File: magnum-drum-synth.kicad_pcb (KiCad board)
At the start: 2 copper layers, 143.8 x 103.8 mm, 148 parts, among them J1 Input1, J2 Input1, J3 Trig_In, J4 Freq_CV, J5 Decay_CV, J6 Audio_Out, J7 Euro_Power, Q1 2N3904, Q2 2N3904, Q3 2N3904, Q4 2N3906, Q5 2N3906, Q6 2N3906, SW1 SW_SPDT, U1 HEF4093B, U2 TL072, U3 TL074, U4 LM13700, U5 LM13700, U6 LM13700

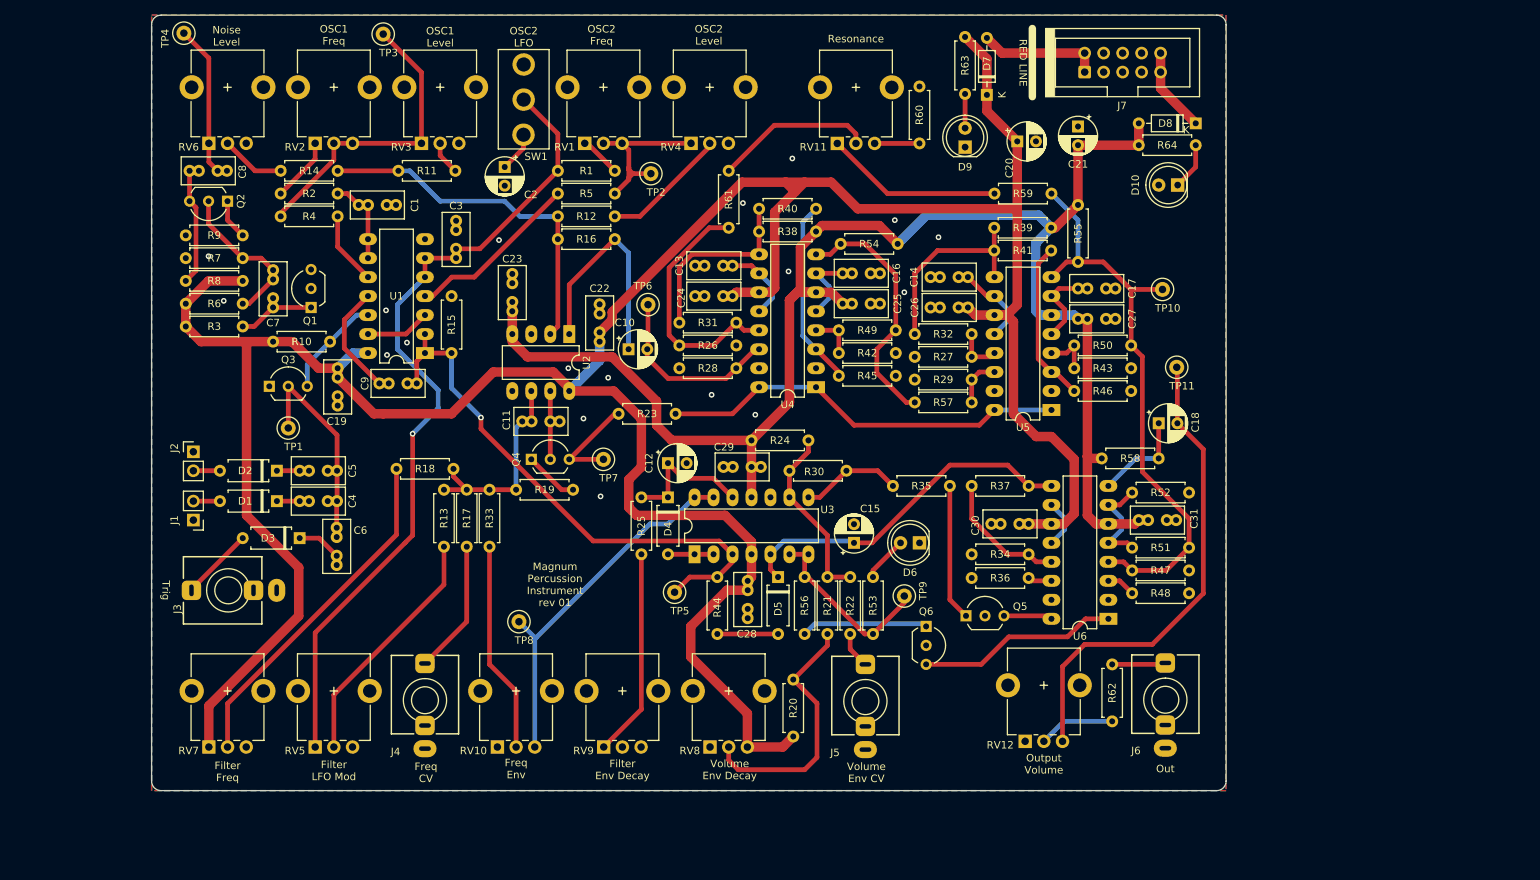
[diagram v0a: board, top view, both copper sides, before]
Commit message: Creating rev02
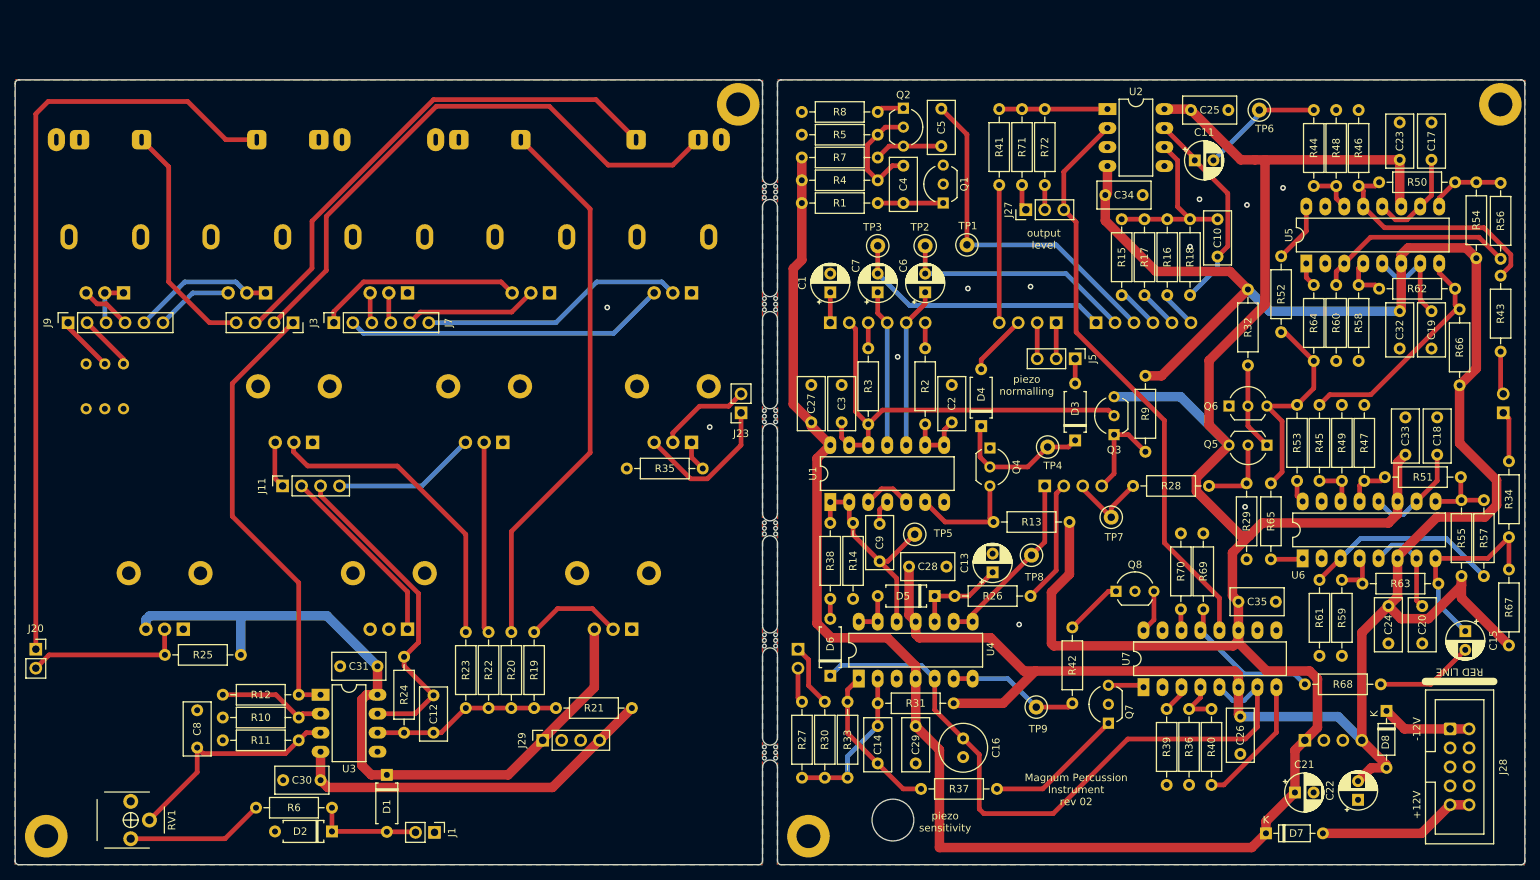
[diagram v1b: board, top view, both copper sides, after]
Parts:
- removed D10, D9: LED, LED_THT:LED_D5.0mm
- removed TP10, TP11: TestPoint, TestPoint:TestPoint_Loop_D2.50mm_Drill1.0mm_LowProfile
- added C32: 100nF (X7R), Rumblesan_Footprints:C_Rect_L7.0mm_W3.5mm_P5.00mm, F.Cu at (215.3, 65.9)
- added C33: 100nF (X7R), Rumblesan_Footprints:C_Rect_L7.0mm_W3.5mm_P5.00mm, F.Cu at (216.0, 80.2)
- added C34: 100nF (X7R), Rumblesan_Footprints:C_Rect_L7.0mm_W3.5mm_P5.00mm, F.Cu at (180.9, 45.4)
- added C35: 100nF (X7R), Rumblesan_Footprints:C_Rect_L7.0mm_W3.5mm_P5.00mm, F.Cu at (193.7, 99.8)
- added H1: MouseBite, Panelization:mouse-bite-2mm-slot, F.Cu at (131.0, 105.0)
- added H10: MountingHole_Pad, MountingHole:MountingHole_3.2mm_M3_ISO7380_Pad, F.Cu at (126.7, 33.3)
- added H2: MouseBite, Panelization:mouse-bite-2mm-slot, F.Cu at (131.0, 45.0)
- added H3: MouseBite, Panelization:mouse-bite-2mm-slot, F.Cu at (131.0, 75.0)
- added H4: MouseBite, Panelization:mouse-bite-2mm-slot, F.Cu at (131.0, 60.0)
- added H5: MouseBite, Panelization:mouse-bite-2mm-slot, F.Cu at (131.0, 120.0)
- added H6: MouseBite, Panelization:mouse-bite-2mm-slot, F.Cu at (131.0, 90.0)
- added H7: MountingHole_Pad, MountingHole:MountingHole_3.2mm_M3_ISO7380_Pad, F.Cu at (228.7, 33.3)
- added H8: MountingHole_Pad, MountingHole:MountingHole_3.2mm_M3_ISO7380_Pad, F.Cu at (136.1, 131.2)
- added H9: MountingHole_Pad, MountingHole:MountingHole_3.2mm_M3_ISO7380_Pad, F.Cu at (34.2, 131.2)
- added J10: Filter_Mod_Main, Connector_PinSocket_2.54mm:PinSocket_1x04_P2.54mm_Vertical, B.Cu at (167.8, 84.3)
- added J11: Filter_Mod_Ctrl, Connector_PinSocket_2.54mm:PinSocket_1x04_P2.54mm_Vertical, F.Cu at (65.8, 84.3)
- added J12: Freq_CV, EurorackBasics:Jack_3.5mm_QingPu_WQP-PJ398SM_Vertical, B.Cu at (92.8, 38.0)
- added J18: Decay_CV, EurorackBasics:Jack_3.5mm_QingPu_WQP-PJ398SM_Vertical, B.Cu at (67.2, 38.0)
- added J20: Amp_Decay_Ctrl, Connector_PinSocket_2.54mm:PinSocket_1x02_P2.54mm_Vertical, F.Cu at (32.8, 106.2)
- added J21: Amp_Decay_Main, Connector_PinHeader_2.54mm:PinHeader_1x02_P2.54mm_Vertical, B.Cu at (134.7, 106.2)
- added J22: Res_Main, Connector_PinHeader_2.54mm:PinHeader_1x02_P2.54mm_Vertical, B.Cu at (229.1, 74.5)
- added J23: Res_Ctrl, Connector_PinSocket_2.54mm:PinSocket_1x02_P2.54mm_Vertical, F.Cu at (127.1, 74.5)
- added J26: Audio_Out, EurorackBasics:Jack_3.5mm_QingPu_WQP-PJ398SM_Vertical, B.Cu at (42.0, 38.0)
- added J27: LevelSelect, Connector_PinHeader_2.54mm:PinHeader_1x03_P2.54mm_Vertical, F.Cu at (165.2, 47.4)
- added J28: Eurorack_Power_Small, EurorackBasics:Eurorack_PowerHeader_2x05_P2.54mm_Shrouded, F.Cu at (222.0, 116.8)
- added J29: POWER_CTRL, Connector_PinSocket_2.54mm:PinSocket_1x04_P2.54mm_Vertical, F.Cu at (100.6, 118.4)
- added J30: POWER_MAIN, Connector_PinHeader_2.54mm:PinHeader_1x04_P2.54mm_Vertical, B.Cu at (202.6, 118.4)
- added J8: Osc_Freq_Main, Connector_PinHeader_2.54mm:PinHeader_1x06_P2.54mm_Vertical, B.Cu at (139.1, 62.5)
- added J9: Osc_Freq_Ctrl, Connector_PinSocket_2.54mm:PinSocket_1x06_P2.54mm_Vertical, F.Cu at (37.1, 62.5)
- added Q7: 2N3906, Package_TO_SOT_THT:TO-92_Inline_Wide, F.Cu at (176.3, 116.1)
- added Q8: 2N3906, Package_TO_SOT_THT:TO-92_Inline_Wide, F.Cu at (177.3, 98.4)
- added R65: 21k, Rumblesan_Footprints:Resistor_THT_L6.3mm_D2.5mm_P10.16mm_Horizontal, F.Cu at (198.0, 94.1)
- added R66: 10k, Rumblesan_Footprints:Resistor_THT_L6.3mm_D2.5mm_P10.16mm_Horizontal, F.Cu at (223.3, 60.7)
- added R67: 10k, Rumblesan_Footprints:Resistor_THT_L6.3mm_D2.5mm_P10.16mm_Horizontal, F.Cu at (229.9, 95.5)
- added R68: 100k, Rumblesan_Footprints:Resistor_THT_L6.3mm_D2.5mm_P10.16mm_Horizontal, F.Cu at (212.7, 110.9)
- added R69: 220r, Rumblesan_Footprints:Resistor_THT_L6.3mm_D2.5mm_P10.16mm_Horizontal, F.Cu at (189.0, 100.8)
- added R70: 220r, Rumblesan_Footprints:Resistor_THT_L6.3mm_D2.5mm_P10.16mm_Horizontal, F.Cu at (186.0, 100.8)
- added R71: 18k, Rumblesan_Footprints:Resistor_THT_L6.3mm_D2.5mm_P10.16mm_Horizontal, F.Cu at (164.7, 44.1)
- added R72: 4k7, Rumblesan_Footprints:Resistor_THT_L6.3mm_D2.5mm_P10.16mm_Horizontal, F.Cu at (167.8, 44.1)
- added U7: LM13700, Package_DIP:DIP-16_W7.62mm_LongPads, F.Cu at (181.0, 111.3)
- C1, C7: value 47nF -> 1uF; footprint Rumblesan_Footprints:C_Rect_L7.0mm_W3.5mm_P2.50mm_P5.00mm -> Capacitor_THT:CP_Radial_D5.0mm_P2.50mm
- C10: value 10uF -> 22pF; footprint Capacitor_THT:CP_Radial_D5.0mm_P2.50mm -> Rumblesan_Footprints:C_Rect_L7.0mm_W3.5mm_P5.00mm
- C11: value 47pF -> 10uF; footprint Rumblesan_Footprints:C_Rect_L7.0mm_W3.5mm_P2.50mm_P5.00mm -> Capacitor_THT:CP_Radial_D5.0mm_P2.50mm
- C12: value 10uF -> 10nF; footprint Capacitor_THT:CP_Radial_D5.0mm_P2.50mm -> Rumblesan_Footprints:C_Rect_L7.0mm_W3.5mm_P5.00mm
- C13: value 1nF -> 10uF; footprint Rumblesan_Footprints:C_Rect_L7.0mm_W3.5mm_P2.50mm_P5.00mm -> Capacitor_THT:CP_Radial_D5.0mm_P2.50mm
- C14: value 1nF -> 22pF; footprint Rumblesan_Footprints:C_Rect_L7.0mm_W3.5mm_P2.50mm_P5.00mm -> Rumblesan_Footprints:C_Rect_L7.0mm_W3.5mm_P5.00mm
- C15: value 1uF -> 10uF
- C16: value 1nF -> 1uF; footprint Rumblesan_Footprints:C_Rect_L7.0mm_W3.5mm_P2.50mm_P5.00mm -> Capacitor_THT:C_Radial_D6.3mm_H7.0mm_P2.50mm
- C17: value 1nF -> 150pF (poly); footprint Rumblesan_Footprints:C_Rect_L7.0mm_W3.5mm_P2.50mm_P5.00mm -> Rumblesan_Footprints:C_Rect_L7.0mm_W3.5mm_P5.00mm
- C18: value 10uF -> 150pF (poly); footprint Capacitor_THT:CP_Radial_D5.0mm_P2.50mm -> Rumblesan_Footprints:C_Rect_L7.0mm_W3.5mm_P5.00mm
- C19: value 100nF (X7R) -> 150pF (poly); footprint Rumblesan_Footprints:C_Rect_L7.0mm_W3.5mm_P2.50mm_P5.00mm -> Rumblesan_Footprints:C_Rect_L7.0mm_W3.5mm_P5.00mm
- C2: value 1uF -> 47nF; footprint Capacitor_THT:CP_Radial_D5.0mm_P2.50mm -> Rumblesan_Footprints:C_Rect_L7.0mm_W3.5mm_P5.00mm
- C20: value 1uF -> 150pF (poly); footprint Capacitor_THT:CP_Radial_D5.0mm_P2.50mm -> Rumblesan_Footprints:C_Rect_L7.0mm_W3.5mm_P5.00mm
- C22: value 100nF (X7R) -> 1uF; footprint Rumblesan_Footprints:C_Rect_L7.0mm_W3.5mm_P2.50mm_P5.00mm -> Capacitor_THT:CP_Radial_D5.0mm_P2.50mm
- C23, C24, C25, C26, C27, C28, C29, C3, C30, C31, C5: footprint Rumblesan_Footprints:C_Rect_L7.0mm_W3.5mm_P2.50mm_P5.00mm -> Rumblesan_Footprints:C_Rect_L7.0mm_W3.5mm_P5.00mm
- C4: value 100nF -> 47nF; footprint Rumblesan_Footprints:C_Rect_L7.0mm_W3.5mm_P2.50mm_P5.00mm -> Rumblesan_Footprints:C_Rect_L7.0mm_W3.5mm_P5.00mm
- C6: value 100nF -> 1uF; footprint Rumblesan_Footprints:C_Rect_L7.0mm_W3.5mm_P2.50mm_P5.00mm -> Capacitor_THT:CP_Radial_D5.0mm_P2.50mm
- C8, C9: value 100nF -> 220nF; footprint Rumblesan_Footprints:C_Rect_L7.0mm_W3.5mm_P2.50mm_P5.00mm -> Rumblesan_Footprints:C_Rect_L7.0mm_W3.5mm_P5.00mm
- D1, D2, D3, D4, D5: value D -> 1n4148
- D6: value LED -> 1n4148; footprint LED_THT:LED_D5.0mm -> Rumblesan_Footprints:Diode_THT_P7.62mm_Horizontal
- D7, D8: value 1N5189 -> 1N5818
- J1: value Input1 -> Piezo
- J2: value Input1 -> Trig_In; footprint Connector_PinHeader_2.54mm:PinHeader_1x02_P2.54mm_Vertical -> EurorackBasics:Jack_3.5mm_QingPu_WQP-PJ398SM_Vertical; moved to B.Cu
- J3: value Trig_In -> Trig_Ctrl; footprint AudioJacks:Jack_3.5mm_QingPu_WQP-PJ398SM_Vertical -> Connector_PinSocket_2.54mm:PinSocket_1x04_P2.54mm_Vertical
- J4: value Freq_CV -> Trig_Main; footprint AudioJacks:Jack_3.5mm_QingPu_WQP-PJ398SM_Vertical -> Connector_PinHeader_2.54mm:PinHeader_1x04_P2.54mm_Vertical; moved to B.Cu
- J5: value Decay_CV -> Tap_Normal; footprint AudioJacks:Jack_3.5mm_QingPu_WQP-PJ398SM_Vertical -> Connector_PinHeader_2.54mm:PinHeader_1x03_P2.54mm_Vertical
- J6: value Audio_Out -> Signals_Main; footprint AudioJacks:Jack_3.5mm_QingPu_WQP-PJ398SM_Vertical -> Connector_PinSocket_2.54mm:PinSocket_1x06_P2.54mm_Vertical; moved to B.Cu
- J7: value Euro_Power -> Signals_Main; footprint EurorackBasics:EurorackPowerHeader_2x05_P2.54mm_Shrouded -> Connector_PinSocket_2.54mm:PinSocket_1x06_P2.54mm_Vertical
- Q4, Q5: value 2N3906 -> 2N3904
- R1: value 22k -> 100k; footprint Resistor_THT:R_Axial_DIN0207_L6.3mm_D2.5mm_P7.62mm_Horizontal -> Rumblesan_Footprints:Resistor_THT_L6.3mm_D2.5mm_P10.16mm_Horizontal
- R10: value R -> 10k; footprint Resistor_THT:R_Axial_DIN0207_L6.3mm_D2.5mm_P7.62mm_Horizontal -> Rumblesan_Footprints:Resistor_THT_L6.3mm_D2.5mm_P10.16mm_Horizontal
- R11: value 100k -> 1m; footprint Resistor_THT:R_Axial_DIN0207_L6.3mm_D2.5mm_P7.62mm_Horizontal -> Rumblesan_Footprints:Resistor_THT_L6.3mm_D2.5mm_P10.16mm_Horizontal
- R12: value 100k -> 220k; footprint Resistor_THT:R_Axial_DIN0207_L6.3mm_D2.5mm_P7.62mm_Horizontal -> Rumblesan_Footprints:Resistor_THT_L6.3mm_D2.5mm_P10.16mm_Horizontal
- R13: value 100k -> 10k; footprint Resistor_THT:R_Axial_DIN0207_L6.3mm_D2.5mm_P7.62mm_Horizontal -> Rumblesan_Footprints:Resistor_THT_L6.3mm_D2.5mm_P10.16mm_Horizontal
- R14, R16, R17, R18, R19, R2, R22, R23, R31, R32, R36, R40, R46, R47, R48, R50, R51, R54, R55, R57: footprint Resistor_THT:R_Axial_DIN0207_L6.3mm_D2.5mm_P7.62mm_Horizontal -> Rumblesan_Footprints:Resistor_THT_L6.3mm_D2.5mm_P10.16mm_Horizontal
- R15, R44, R56: value R -> 100k; footprint Resistor_THT:R_Axial_DIN0207_L6.3mm_D2.5mm_P7.62mm_Horizontal -> Rumblesan_Footprints:Resistor_THT_L6.3mm_D2.5mm_P10.16mm_Horizontal
- R20: value 15k -> 100k; footprint Resistor_THT:R_Axial_DIN0207_L6.3mm_D2.5mm_P7.62mm_Horizontal -> Rumblesan_Footprints:Resistor_THT_L6.3mm_D2.5mm_P10.16mm_Horizontal
- R21: value 120k -> 150k; footprint Resistor_THT:R_Axial_DIN0207_L6.3mm_D2.5mm_P7.62mm_Horizontal -> Rumblesan_Footprints:Resistor_THT_L6.3mm_D2.5mm_P10.16mm_Horizontal
- R24: value 100k -> 2k; footprint Resistor_THT:R_Axial_DIN0207_L6.3mm_D2.5mm_P7.62mm_Horizontal -> Rumblesan_Footprints:Resistor_THT_L6.3mm_D2.5mm_P10.16mm_Horizontal
- R25: value R -> 15k; footprint Resistor_THT:R_Axial_DIN0207_L6.3mm_D2.5mm_P7.62mm_Horizontal -> Rumblesan_Footprints:Resistor_THT_L6.3mm_D2.5mm_P10.16mm_Horizontal
- R26: value 220r -> 1k; footprint Resistor_THT:R_Axial_DIN0207_L6.3mm_D2.5mm_P7.62mm_Horizontal -> Rumblesan_Footprints:Resistor_THT_L6.3mm_D2.5mm_P10.16mm_Horizontal
- R27: value 220r -> 120k; footprint Resistor_THT:R_Axial_DIN0207_L6.3mm_D2.5mm_P7.62mm_Horizontal -> Rumblesan_Footprints:Resistor_THT_L6.3mm_D2.5mm_P10.16mm_Horizontal
- R28: value 220r -> 51r; footprint Resistor_THT:R_Axial_DIN0207_L6.3mm_D2.5mm_P7.62mm_Horizontal -> Rumblesan_Footprints:Resistor_THT_L6.3mm_D2.5mm_P10.16mm_Horizontal
- R29: value 220r -> 470r; footprint Resistor_THT:R_Axial_DIN0207_L6.3mm_D2.5mm_P7.62mm_Horizontal -> Rumblesan_Footprints:Resistor_THT_L6.3mm_D2.5mm_P10.16mm_Horizontal
- R3: value 100k -> 22k; footprint Resistor_THT:R_Axial_DIN0207_L6.3mm_D2.5mm_P7.62mm_Horizontal -> Rumblesan_Footprints:Resistor_THT_L6.3mm_D2.5mm_P10.16mm_Horizontal
- R30: value 27k -> 100k; footprint Resistor_THT:R_Axial_DIN0207_L6.3mm_D2.5mm_P7.62mm_Horizontal -> Rumblesan_Footprints:Resistor_THT_L6.3mm_D2.5mm_P10.16mm_Horizontal
- R33: value 100k -> 27k; footprint Resistor_THT:R_Axial_DIN0207_L6.3mm_D2.5mm_P7.62mm_Horizontal -> Rumblesan_Footprints:Resistor_THT_L6.3mm_D2.5mm_P10.16mm_Horizontal
- R34: value 470r -> 20k; footprint Resistor_THT:R_Axial_DIN0207_L6.3mm_D2.5mm_P7.62mm_Horizontal -> Rumblesan_Footprints:Resistor_THT_L6.3mm_D2.5mm_P10.16mm_Horizontal
- R35: value 4k3 -> 2k; footprint Resistor_THT:R_Axial_DIN0207_L6.3mm_D2.5mm_P7.62mm_Horizontal -> Rumblesan_Footprints:Resistor_THT_L6.3mm_D2.5mm_P10.16mm_Horizontal
- R37: value 100k -> 4k3; footprint Resistor_THT:R_Axial_DIN0207_L6.3mm_D2.5mm_P7.62mm_Horizontal -> Rumblesan_Footprints:Resistor_THT_L6.3mm_D2.5mm_P10.16mm_Horizontal
- R38: value 10k -> 680r; footprint Resistor_THT:R_Axial_DIN0207_L6.3mm_D2.5mm_P7.62mm_Horizontal -> Rumblesan_Footprints:Resistor_THT_L6.3mm_D2.5mm_P10.16mm_Horizontal
- R39: value 10k -> 470r; footprint Resistor_THT:R_Axial_DIN0207_L6.3mm_D2.5mm_P7.62mm_Horizontal -> Rumblesan_Footprints:Resistor_THT_L6.3mm_D2.5mm_P10.16mm_Horizontal
- R4: value 100r -> 1m; footprint Resistor_THT:R_Axial_DIN0207_L6.3mm_D2.5mm_P7.62mm_Horizontal -> Rumblesan_Footprints:Resistor_THT_L6.3mm_D2.5mm_P10.16mm_Horizontal
- R41: value 100k -> 1k; footprint Resistor_THT:R_Axial_DIN0207_L6.3mm_D2.5mm_P7.62mm_Horizontal -> Rumblesan_Footprints:Resistor_THT_L6.3mm_D2.5mm_P10.16mm_Horizontal
- R42: value 220r -> 33k; footprint Resistor_THT:R_Axial_DIN0207_L6.3mm_D2.5mm_P7.62mm_Horizontal -> Rumblesan_Footprints:Resistor_THT_L6.3mm_D2.5mm_P10.16mm_Horizontal
- R43: value 220r -> 6k8; footprint Resistor_THT:R_Axial_DIN0207_L6.3mm_D2.5mm_P7.62mm_Horizontal -> Rumblesan_Footprints:Resistor_THT_L6.3mm_D2.5mm_P10.16mm_Horizontal
- R45: value 220r -> 100k; footprint Resistor_THT:R_Axial_DIN0207_L6.3mm_D2.5mm_P7.62mm_Horizontal -> Rumblesan_Footprints:Resistor_THT_L6.3mm_D2.5mm_P10.16mm_Horizontal
- R49: value 100k -> 220r; footprint Resistor_THT:R_Axial_DIN0207_L6.3mm_D2.5mm_P7.62mm_Horizontal -> Rumblesan_Footprints:Resistor_THT_L6.3mm_D2.5mm_P10.16mm_Horizontal
- R5: value 100r -> 100k; footprint Resistor_THT:R_Axial_DIN0207_L6.3mm_D2.5mm_P7.62mm_Horizontal -> Rumblesan_Footprints:Resistor_THT_L6.3mm_D2.5mm_P10.16mm_Horizontal
- R52: value 10k -> 21k; footprint Resistor_THT:R_Axial_DIN0207_L6.3mm_D2.5mm_P7.62mm_Horizontal -> Rumblesan_Footprints:Resistor_THT_L6.3mm_D2.5mm_P10.16mm_Horizontal
- R53: value R -> 21k; footprint Resistor_THT:R_Axial_DIN0207_L6.3mm_D2.5mm_P7.62mm_Horizontal -> Rumblesan_Footprints:Resistor_THT_L6.3mm_D2.5mm_P10.16mm_Horizontal
- R58, R59: value 10k -> 220r; footprint Resistor_THT:R_Axial_DIN0207_L6.3mm_D2.5mm_P7.62mm_Horizontal -> Rumblesan_Footprints:Resistor_THT_L6.3mm_D2.5mm_P10.16mm_Horizontal
- R6: value 1m -> 10k; footprint Resistor_THT:R_Axial_DIN0207_L6.3mm_D2.5mm_P7.62mm_Horizontal -> Rumblesan_Footprints:Resistor_THT_L6.3mm_D2.5mm_P10.16mm_Horizontal
- R60: value 1k -> 220r; footprint Resistor_THT:R_Axial_DIN0207_L6.3mm_D2.5mm_P7.62mm_Horizontal -> Rumblesan_Footprints:Resistor_THT_L6.3mm_D2.5mm_P10.16mm_Horizontal
- R61: value 6k8 -> 220r; footprint Resistor_THT:R_Axial_DIN0207_L6.3mm_D2.5mm_P7.62mm_Horizontal -> Rumblesan_Footprints:Resistor_THT_L6.3mm_D2.5mm_P10.16mm_Horizontal
- R62: value 1k -> 100k; footprint Resistor_THT:R_Axial_DIN0207_L6.3mm_D2.5mm_P7.62mm_Horizontal -> Rumblesan_Footprints:Resistor_THT_L6.3mm_D2.5mm_P10.16mm_Horizontal
- R63: value 3k3 -> 100k; footprint Resistor_THT:R_Axial_DIN0207_L6.3mm_D2.5mm_P7.62mm_Horizontal -> Rumblesan_Footprints:Resistor_THT_L6.3mm_D2.5mm_P10.16mm_Horizontal
- R64: value 3k3 -> 21k; footprint Resistor_THT:R_Axial_DIN0207_L6.3mm_D2.5mm_P7.62mm_Horizontal -> Rumblesan_Footprints:Resistor_THT_L6.3mm_D2.5mm_P10.16mm_Horizontal
- R7: value 100k -> 6k8; footprint Resistor_THT:R_Axial_DIN0207_L6.3mm_D2.5mm_P7.62mm_Horizontal -> Rumblesan_Footprints:Resistor_THT_L6.3mm_D2.5mm_P10.16mm_Horizontal
- R8: value 6k8 -> 22r; footprint Resistor_THT:R_Axial_DIN0207_L6.3mm_D2.5mm_P7.62mm_Horizontal -> Rumblesan_Footprints:Resistor_THT_L6.3mm_D2.5mm_P10.16mm_Horizontal
- R9: value 22r -> 10k; footprint Resistor_THT:R_Axial_DIN0207_L6.3mm_D2.5mm_P7.62mm_Horizontal -> Rumblesan_Footprints:Resistor_THT_L6.3mm_D2.5mm_P10.16mm_Horizontal
- RV1: value 1mA -> 100k; footprint Rumblesan_Footprints:Potentiometer_Alpha_RD901F-40-00D_Single_Vertical_CircularHoles -> Rumblesan_Footprints:Potentiometer_THT_Bourns_3306P_Vertical
- RV10, RV12: moved to B.Cu
- RV11: value 50kA -> 100k; moved to B.Cu
- RV2: value 1mA -> 100kA; footprint Rumblesan_Footprints:Potentiometer_Alpha_RD901F-40-00D_Single_Vertical_CircularHoles -> Rumblesan_Footprints:Potentiometer_Alpha_RD901F-40-00D_Single_Vertical; moved to B.Cu
- RV3, RV4: value 100kA -> 1mA; footprint Rumblesan_Footprints:Potentiometer_Alpha_RD901F-40-00D_Single_Vertical_CircularHoles -> Rumblesan_Footprints:Potentiometer_Alpha_RD901F-40-00D_Single_Vertical; moved to B.Cu
- RV5: value 100kB -> 100kA; footprint Rumblesan_Footprints:Potentiometer_Alpha_RD901F-40-00D_Single_Vertical_CircularHoles -> Rumblesan_Footprints:Potentiometer_Alpha_RD901F-40-00D_Single_Vertical; moved to B.Cu
- RV6: footprint Rumblesan_Footprints:Potentiometer_Alpha_RD901F-40-00D_Single_Vertical_CircularHoles -> Rumblesan_Footprints:Potentiometer_Alpha_RD901F-40-00D_Single_Vertical; moved to B.Cu
- RV7: value 100kB -> 100k; moved to B.Cu
- RV8, RV9: value 100k -> 100kB; moved to B.Cu
- SW1: value SW_SPDT -> SW_DPDT_x2; footprint Rumblesan_Footprints:SW_SPDT_DailyWell_MiniToggle -> Rumblesan_Footprints:SW_PUSH_2P2T_8mm_Apem_MHPS2285; moved to B.Cu
- TP1: value TestPoint -> Noise TestPoint
- TP2: value TestPoint -> OSC1 TestPoint
- TP3: value TestPoint -> OSC2 TestPoint
- TP4: value TestPoint -> Trigger TestPoint
- TP5: value TestPoint -> Schmitt Trigger TestPoint
- TP6: value TestPoint -> Mixer TestPoint
- TP8: value TestPoint -> Filter Env TestPoint
- U3: value TL074 -> TL072; footprint Package_DIP:DIP-14_W7.62mm_LongPads -> Package_DIP:DIP-8_W7.62mm_LongPads
- U4: value LM13700 -> TL074; footprint Package_DIP:DIP-16_W7.62mm_LongPads -> Package_DIP:DIP-14_W7.62mm_LongPads
- moved C19 146.4 mm to (219.5, 65.9), turned to 90 degrees
- moved TP4 128.2 mm to (168.1, 79.1), turned to 0 degrees
- moved R9 124.2 mm to (181.2, 79.8), turned to 90 degrees
- moved C23 119.7 mm to (215.3, 40.7), turned to 90 degrees
- moved C22 118.6 mm to (209.7, 126.3)
- moved RV1 116.7 mm to (45.5, 129.0), turned to -90 degrees
- moved Q3 113.2 mm to (177.0, 77.5), turned to 90 degrees
- moved R18 111.3 mm to (187.2, 48.6), turned to -90 degrees
- moved C31 108.6 mm to (78.5, 108.5)
- moved R56 107.0 mm to (228.8, 43.8)
- moved J7 105.9 mm to (72.6, 62.5)
- moved D7 105.6 mm to (197.4, 130.8), turned to 0 degrees
- moved C30 105.5 mm to (65.9, 123.7), turned to 0 degrees
- moved D3 104.6 mm to (171.8, 78.2), turned to 90 degrees
- moved R44 101.4 mm to (203.8, 34.0)
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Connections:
- C1 pad 1: GND -> /OSC2_LFO_Cap
- C1 pad 2: Net-(C1-Pad2) -> GND
- C11 pad 1: Net-(C11-Pad1) -> Net-(C10-Pad2)
- C11 pad 2: Net-(C11-Pad2) -> /Filter/Input
- C12 pad 2: GND -> /Freq_Control_Ctrl
- C13 pad 1: GND -> Net-(C13-Pad1)
- C13 pad 2: Net-(C13-Pad2) -> GND
- C14 pad 1: GND -> Net-(C14-Pad1)
- C15 pad 1: Net-(C15-Pad1) -> /Filter/Output
- C15 pad 2: GND -> /OutputVCA/Input
- C16 pad 1: GND -> Net-(C16-Pad1)
- C16 pad 2: Net-(C16-Pad2) -> GND
- C18 pad 1: Net-(C18-Pad1) -> GND
- C19 pad 1: +12V -> GND
- C19 pad 2: GND -> Net-(C19-Pad2)
- C2 pad 1: Net-(C2-Pad1) -> GND
- C2 pad 2: GND -> Net-(C2-Pad2)
- C20 pad 1: +12V -> GND
- C20 pad 2: GND -> Net-(C20-Pad2)
- C21 pad 1: GND -> +12V
- C21 pad 2: -12V -> GND
- C22 pad 1: +12V -> GND
- C22 pad 2: GND -> -12V
- C23 pad 1: GND -> +12V
- C23 pad 2: -12V -> GND
- C24 pad 1: +12V -> GND
- C24 pad 2: GND -> -12V
- C25 pad 1: GND -> +12V
- C25 pad 2: -12V -> GND
- C26 pad 1: +12V -> GND
- C26 pad 2: GND -> -12V
- C27 pad 1: GND -> +12V
- C27 pad 2: -12V -> GND
- C28 pad 1: +12V -> GND
- C28 pad 2: GND -> -12V
- C29 pad 1: GND -> +12V
- C29 pad 2: -12V -> GND
- C3 pad 1: GND -> /OSC2_LFO_Main
- C3 pad 2: Net-(C3-Pad2) -> GND
- C30 pad 1: +12V -> GND
- C30 pad 2: GND -> -12V
- C31 pad 1: GND -> +12V
- C31 pad 2: -12V -> GND
- C5 pad 2: Net-(C4-Pad2) -> /Noise_Signal
- C6 pad 1: Net-(C6-Pad1) -> /OSC1_Freq_R
- C6 pad 2: Net-(C4-Pad2) -> /OSC1_Signal
- C7 pad 1: Net-(C7-Pad1) -> /OSC2_Freq_R
- C7 pad 2: Net-(C7-Pad2) -> /OSC2_Signal
- C8 pad 1: Net-(C8-Pad1) -> GND
- C9 pad 2: Net-(C9-Pad2) -> /Trigger
- D1 pad 1: Net-(C4-Pad1) -> +12V
- D2 pad 1: Net-(C5-Pad1) -> Net-(D1-Pad2)
- D2 pad 2: Net-(D2-Pad2) -> GND
- D3 pad 1: Net-(C6-Pad1) -> Net-(D3-Pad1)
- D4 pad 1: Net-(C12-Pad1) -> Net-(D3-Pad1)
- D5 pad 1: Net-(C15-Pad1) -> Net-(C13-Pad1)
- D6 pad 1: GND -> Net-(C16-Pad1)
- J7 pad 1: Net-(D7-Pad2) -> Net-(J7-Pad1)
- J7 pad 2: Net-(D7-Pad2) -> Net-(J7-Pad2)
- J7 pad 3: GND -> Net-(J7-Pad3)
- J7 pad 4: GND -> Net-(J7-Pad4)
- J7 pad 5: GND -> Net-(J7-Pad5)
- J7 pad 6: GND -> Net-(J7-Pad6)
- Q1 pad 1: Net-(C7-Pad1) -> Net-(C4-Pad1)
- Q2 pad 2: Net-(C7-Pad2) -> Net-(C4-Pad2)
- Q2 pad 3: Net-(C8-Pad1) -> Net-(C5-Pad1)
- Q3 pad 1: GND -> /OSC2_LFO_Signal
- Q3 pad 2: Net-(C4-Pad2) -> /OSC2_LFO_Main
- Q3 pad 3: Net-(Q3-Pad3) -> +12V
- Q4 pad 1: Net-(Q4-Pad1) -> GND
- Q4 pad 2: Net-(C11-Pad2) -> Net-(D3-Pad1)
- Q5 pad 2: GND -> Net-(Q5-Pad2)
- Q5 pad 3: Net-(Q5-Pad3) -> +12V
- Q6 pad 1: Net-(Q6-Pad1) -> GND
- Q6 pad 2: GND -> Net-(Q5-Pad1)
- Q6 pad 3: Net-(Q6-Pad3) -> /Filter/I_Freq
- R1 pad 1: Net-(C3-Pad2) -> +12V
- R1 pad 2: Net-(R1-Pad2) -> Net-(C4-Pad1)
- R10 pad 1: +12V -> GND
- R10 pad 2: Net-(Q3-Pad3) -> Net-(R10-Pad2)
- R11 pad 1: Net-(R11-Pad1) -> Net-(C8-Pad2)
- R11 pad 2: Net-(R11-Pad2) -> GND
- R12 pad 1: Net-(R12-Pad1) -> Net-(J3-Pad1)
- R12 pad 2: Net-(R11-Pad2) -> Net-(R10-Pad2)
- R13 pad 1: Net-(R13-Pad1) -> +12V
- R13 pad 2: Net-(C11-Pad1) -> Net-(Q4-Pad3)
- R14 pad 1: Net-(R14-Pad1) -> /Trigger
- R14 pad 2: Net-(R11-Pad2) -> GND
- R15 pad 1: Net-(C9-Pad2) -> /Noise_Return
- R15 pad 2: GND -> Net-(C10-Pad1)
- R16 pad 1: Net-(R11-Pad2) -> /OSC1_Return
- R17 pad 1: Net-(J4-PadT) -> /OSC2_Return
- R17 pad 2: Net-(C11-Pad1) -> Net-(C10-Pad1)
- R18 pad 1: Net-(R18-Pad1) -> Net-(C10-Pad1)
- R18 pad 2: Net-(C11-Pad1) -> Net-(C10-Pad2)
- R19 pad 1: Net-(C11-Pad1) -> Net-(R19-Pad1)
- R19 pad 2: Net-(Q4-Pad1) -> Net-(C12-Pad1)
- R2 pad 1: Net-(C1-Pad2) -> Net-(C2-Pad2)
- R2 pad 2: Net-(R2-Pad2) -> /OSC1_Freq_L
- R20 pad 1: Net-(R20-Pad1) -> Net-(J12-PadT)
- R20 pad 2: +12V -> Net-(C12-Pad1)
- R21 pad 1: Net-(R21-Pad1) -> -12V
- R21 pad 2: Net-(R20-Pad1) -> Net-(C12-Pad1)
- R22 pad 1: Net-(J5-PadT) -> Net-(R22-Pad1)
- R22 pad 2: Net-(R21-Pad1) -> Net-(C12-Pad1)
- R23 pad 1: Net-(Q4-Pad3) -> Net-(R23-Pad1)
- R23 pad 2: /I_FREQ -> Net-(C12-Pad1)
- R24 pad 1: Net-(R21-Pad1) -> Net-(C12-Pad1)
- R24 pad 2: -12V -> /Freq_Control_Ctrl
- R25 pad 1: Net-(C12-Pad1) -> Net-(J20-Pad2)
- R25 pad 2: Net-(R25-Pad2) -> +12V
- R26 pad 1: Net-(R26-Pad1) -> Net-(C13-Pad1)
- R26 pad 2: GND -> /Filter_Env_Decay
- R27 pad 1: Net-(R27-Pad1) -> Net-(C14-Pad1)
- R27 pad 2: GND -> Net-(J21-Pad2)
- R28 pad 1: Net-(C10-Pad2) -> /Freq_Control_Main
- R28 pad 2: GND -> Net-(Q5-Pad2)
- R29 pad 1: Net-(R29-Pad1) -> Net-(Q5-Pad2)
- R3 pad 1: +12V -> /OSC2_LFO_Main
- R3 pad 2: Net-(C7-Pad1) -> /OSC2_Freq_L
- R30 pad 1: Net-(R21-Pad1) -> Net-(J21-Pad1)
- R30 pad 2: Net-(R30-Pad2) -> Net-(C14-Pad1)
- R31 pad 1: Net-(R26-Pad1) -> -12V
- R31 pad 2: Net-(R31-Pad2) -> Net-(C14-Pad1)
- R32 pad 1: Net-(R27-Pad1) -> -12V
- R32 pad 2: Net-(R32-Pad2) -> Net-(Q5-Pad1)
- R33 pad 1: Net-(C11-Pad1) -> Net-(C14-Pad1)
- R33 pad 2: Net-(R33-Pad2) -> Net-(C14-Pad2)
- R34 pad 1: GND -> /Filter/Output
- R34 pad 2: Net-(R34-Pad2) -> /Res_Top
- R35 pad 1: Net-(R30-Pad2) -> Net-(R35-Pad1)
- R35 pad 2: Net-(Q5-Pad1) -> GND
- R37 pad 1: Net-(R34-Pad2) -> Net-(C14-Pad2)
- R37 pad 2: Net-(C15-Pad1) -> Net-(Q7-Pad1)
- R38 pad 1: Net-(R31-Pad2) -> /Trigger
- R38 pad 2: -12V -> Net-(D6-Pad2)
- R39 pad 1: Net-(R32-Pad2) -> GND
- R39 pad 2: -12V -> Net-(R39-Pad2)
- R4 pad 1: Net-(R4-Pad1) -> +12V
- R4 pad 2: Net-(R4-Pad2) -> Net-(C4-Pad2)
- R40 pad 1: Net-(R31-Pad2) -> Net-(R36-Pad2)
- R41 pad 1: Net-(R32-Pad2) -> /OutputVCA/Output
- R41 pad 2: Net-(R41-Pad2) -> /Final_Output_Main
- R42 pad 2: GND -> Net-(Q8-Pad1)
- R43 pad 1: Net-(R43-Pad1) -> /Res_Amount
- R43 pad 2: GND -> Net-(R43-Pad2)
- R44 pad 1: Net-(C9-Pad2) -> /Filter/Input
- R44 pad 2: Net-(D5-Pad2) -> Net-(R44-Pad2)
- R45 pad 1: Net-(R40-Pad2) -> Net-(R45-Pad1)
- R45 pad 2: GND -> Net-(R45-Pad2)
- R46 pad 1: Net-(R41-Pad2) -> Net-(R43-Pad2)
- R48 pad 1: Net-(R48-Pad1) -> Net-(R44-Pad2)
- R49 pad 1: Net-(R42-Pad1) -> Net-(R45-Pad2)
- R49 pad 2: Net-(R49-Pad2) -> GND
- R5 pad 1: Net-(R5-Pad1) -> Net-(C4-Pad2)
- R5 pad 2: Net-(R5-Pad2) -> GND
- R50 pad 1: Net-(R43-Pad1) -> Net-(R43-Pad2)
- R50 pad 2: Net-(R47-Pad1) -> Net-(R50-Pad2)
- R52 pad 1: Net-(R51-Pad2) -> Net-(R52-Pad1)
- R52 pad 2: GND -> /Filter/I_Freq
- R53 pad 2: Net-(D6-Pad2) -> /Filter/I_Freq
- R54 pad 1: Net-(R49-Pad2) -> Net-(R50-Pad2)
- R55 pad 1: Net-(R47-Pad1) -> Net-(R51-Pad2)
- R56 pad 1: Net-(R53-Pad1) -> Net-(R50-Pad2)
- R56 pad 2: Net-(Q6-Pad1) -> Net-(R56-Pad2)
- R57 pad 1: Net-(R49-Pad2) -> Net-(R51-Pad2)
- R57 pad 2: Net-(R29-Pad1) -> Net-(R57-Pad2)
- R58 pad 1: Net-(C18-Pad1) -> Net-(R58-Pad1)
- R58 pad 2: -12V -> GND
- R59 pad 1: Net-(R47-Pad1) -> Net-(R59-Pad1)
- R59 pad 2: Net-(R59-Pad2) -> GND
- R6 pad 1: +12V -> Net-(D1-Pad2)
- R6 pad 2: Net-(C7-Pad2) -> Net-(R6-Pad2)
- R60 pad 1: Net-(R60-Pad1) -> Net-(R56-Pad2)
- R61 pad 1: Net-(R26-Pad1) -> Net-(R57-Pad2)
- R61 pad 2: Net-(R61-Pad2) -> GND
- R62 pad 1: Net-(R62-Pad1) -> Net-(R58-Pad1)
- R62 pad 2: Net-(J6-PadT) -> Net-(R45-Pad1)
- R63 pad 1: +12V -> Net-(R59-Pad1)
- R63 pad 2: Net-(D9-Pad2) -> /Filter/Output
- R64 pad 1: Net-(D10-Pad1) -> Net-(R64-Pad1)
- R64 pad 2: -12V -> /Filter/I_Freq
- R7 pad 1: Net-(C7-Pad2) -> +12V
- R7 pad 2: GND -> Net-(C5-Pad1)
- R8 pad 1: +12V -> Net-(Q2-Pad1)
- R8 pad 2: Net-(C8-Pad1) -> GND
- R9 pad 1: Net-(Q2-Pad1) -> /OSC2_LFO_Signal
- R9 pad 2: GND -> -12V
- RV1 pad 1: Net-(R1-Pad2) -> GND
- RV1 pad 2: Net-(R5-Pad2) -> Net-(C8-Pad2)
- RV1 pad 3: Net-(R5-Pad2) -> Net-(R6-Pad2)
- RV10 pad 2: Net-(R33-Pad2) -> Net-(J20-Pad2)
- RV10 pad 3: Net-(RV10-Pad3) -> +12V
- RV11 pad 1: Net-(R59-Pad2) -> /Filter_Env_Decay_Ctrl
- RV11 pad 2: Net-(R61-Pad2) -> GND
- RV11 pad 3: Net-(R60-Pad1) -> GND
- RV12 pad 1: GND -> Net-(R35-Pad1)
- RV12 pad 2: Net-(R62-Pad1) -> Net-(J23-Pad2)
- RV12 pad 3: Net-(C18-Pad2) -> Net-(J23-Pad1)
- RV2 pad 1: Net-(R2-Pad2) -> GND
- RV2 pad 2: Net-(R4-Pad2) -> Net-(J7-Pad5)
- RV2 pad 3: Net-(R4-Pad2) -> Net-(J7-Pad1)
- RV3 pad 1: Net-(R4-Pad2) -> Net-(J9-Pad5)
- RV3 pad 2: Net-(R11-Pad1) -> Net-(J9-Pad5)
- RV3 pad 3: GND -> Net-(J9-Pad6)
- RV4 pad 1: Net-(R5-Pad2) -> Net-(J9-Pad3)
- RV4 pad 2: Net-(R12-Pad1) -> Net-(J9-Pad3)
- RV4 pad 3: GND -> Net-(J9-Pad4)
- RV5 pad 1: Net-(C3-Pad2) -> GND
- RV5 pad 2: Net-(R13-Pad1) -> Net-(J7-Pad6)
- RV5 pad 3: GND -> Net-(J7-Pad2)
- RV6 pad 1: Net-(C8-Pad2) -> GND
- RV6 pad 2: Net-(R14-Pad1) -> Net-(J7-Pad4)
- RV6 pad 3: GND -> Net-(J7-Pad3)
- RV7 pad 1: +12V -> GND
- RV7 pad 2: Net-(R18-Pad1) -> Net-(R23-Pad1)
- RV7 pad 3: GND -> /Filter_Env_Mod_Ctrl
- RV8 pad 2: Net-(R20-Pad1) -> Net-(R19-Pad1)
- RV9 pad 1: Net-(R25-Pad2) -> GND
- RV9 pad 2: GND -> Net-(R22-Pad1)
- RV9 pad 3: GND -> Net-(J11-Pad4)
- SW1 pad 1: Net-(C2-Pad1) -> Net-(J9-Pad1)
- SW1 pad 2: Net-(C3-Pad2) -> Net-(J9-Pad2)
- TP1 pad 1: Net-(C4-Pad2) -> /Noise_Signal
- TP2 pad 1: Net-(R5-Pad2) -> /OSC1_Signal
- TP3 pad 1: Net-(R4-Pad2) -> /OSC2_Signal
- TP4 pad 1: Net-(C8-Pad2) -> Net-(D3-Pad1)
- TP5 pad 1: Net-(C9-Pad2) -> /Trigger
- TP6 pad 1: Net-(C10-Pad2) -> /Filter/Input
- TP7 pad 1: Net-(Q4-Pad3) -> /Freq_Control_Main
- TP8 pad 1: Net-(RV10-Pad3) -> /Filter_Env
- TP9 pad 1: Net-(R53-Pad1) -> Net-(R42-Pad1)
- U1 pad 1: Net-(C9-Pad2) -> /Trigger
- U1 pad 10: Net-(R4-Pad1) -> /OSC1_Freq_R
- U1 pad 11: Net-(C9-Pad1) -> /OSC2_Freq_R
- U1 pad 12: Net-(Q3-Pad3) -> /OSC2_LFO_Main
- U1 pad 13: Net-(U1-Pad13) -> /OSC2_LFO_Main
- U1 pad 2: Net-(C9-Pad2) -> /Trigger
- U1 pad 3: Net-(U1-Pad13) -> Net-(U1-Pad3)
- U1 pad 4: Net-(R5-Pad1) -> Net-(C9-Pad1)
- U1 pad 5: Net-(C3-Pad2) -> Net-(U1-Pad3)
- U1 pad 6: Net-(C3-Pad2) -> Net-(Q4-Pad3)
- U1 pad 8: Net-(C1-Pad2) -> Net-(C2-Pad2)
- U1 pad 9: Net-(C1-Pad2) -> Net-(C2-Pad2)
- U2 pad 1: Net-(C10-Pad1) -> /OutputVCA/Output
- U2 pad 2: Net-(R11-Pad2) -> Net-(J27-Pad3)
- U2 pad 6: Net-(C11-Pad1) -> Net-(C10-Pad1)
- U2 pad 7: Net-(C11-Pad2) -> Net-(C10-Pad2)
- U3 pad 1: Net-(D4-Pad2) -> Net-(J3-Pad1)
- U3 pad 2: Net-(D4-Pad2) -> Net-(R10-Pad2)
- U3 pad 3: Net-(C9-Pad2) -> Net-(C8-Pad2)
- U3 pad 4: +12V -> -12V
- U3 pad 5: Net-(C15-Pad1) -> GND
- U3 pad 6: Net-(R53-Pad1) -> Net-(C12-Pad1)
- U3 pad 7: Net-(R53-Pad1) -> /Freq_Control_Ctrl
- U3 pad 8: Net-(R30-Pad2) -> +12V
- U4 pad 1: /I_FREQ -> Net-(C14-Pad2)
- U4 pad 10: Net-(C13-Pad2) -> Net-(C13-Pad1)
- U4 pad 11: +12V -> -12V
- U4 pad 12: Net-(C13-Pad2) -> /Trigger
- U4 pad 13: Net-(R26-Pad1) -> Net-(D5-Pad2)
- U4 pad 14: Net-(C10-Pad2) -> Net-(D5-Pad2)
- U4 pad 2: unconnected-(U4-Pad2) -> Net-(C14-Pad1)
- U4 pad 3: Net-(R40-Pad2) -> GND
- U4 pad 4: Net-(R42-Pad1) -> +12V
- U4 pad 5: Net-(C16-Pad2) -> Net-(C16-Pad1)
- U4 pad 6: -12V -> Net-(R42-Pad1)
- U4 pad 7: Net-(C16-Pad2) -> Net-(R42-Pad1)
- U4 pad 8: Net-(R49-Pad2) -> /Filter_Env
- U4 pad 9: Net-(R31-Pad2) -> /Filter_Env
- U5 pad 1: /I_FREQ -> Net-(R64-Pad1)
- U5 pad 10: Net-(C14-Pad2) -> Net-(C17-Pad2)
- U5 pad 12: Net-(C14-Pad2) -> Net-(C17-Pad2)
- U5 pad 13: Net-(R27-Pad1) -> Net-(R43-Pad2)
- U5 pad 14: Net-(R29-Pad1) -> Net-(R44-Pad2)
- U5 pad 16: /I_FREQ -> Net-(R52-Pad1)
- U5 pad 3: Net-(R41-Pad2) -> Net-(R56-Pad2)
- U5 pad 4: Net-(R43-Pad1) -> Net-(R58-Pad1)
- U5 pad 5: Net-(C17-Pad2) -> Net-(C19-Pad2)
- U5 pad 7: Net-(C17-Pad2) -> Net-(C19-Pad2)
- U5 pad 8: Net-(R47-Pad1) -> Net-(R45-Pad1)
- U5 pad 9: Net-(R32-Pad2) -> Net-(R50-Pad2)
- U6 pad 1: Net-(Q6-Pad3) -> Net-(R65-Pad1)
- U6 pad 10: Net-(U6-Pad10) -> Net-(C18-Pad2)
- U6 pad 12: Net-(U6-Pad10) -> Net-(C18-Pad2)
- U6 pad 13: Net-(R34-Pad2) -> Net-(R47-Pad1)
- U6 pad 14: Net-(R36-Pad2) -> Net-(R45-Pad2)
- U6 pad 16: Net-(Q5-Pad3) -> Net-(R53-Pad1)
- U6 pad 3: Net-(R48-Pad1) -> Net-(R57-Pad2)
- U6 pad 4: Net-(R47-Pad1) -> Net-(R59-Pad1)
- U6 pad 5: Net-(R51-Pad2) -> Net-(C20-Pad2)
- U6 pad 7: Net-(R51-Pad2) -> Net-(C20-Pad2)
- U6 pad 8: Net-(C18-Pad1) -> /Filter/Output
- U6 pad 9: Net-(C15-Pad1) -> Net-(R51-Pad2)
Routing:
- net -12V: track 212.2 -> 343.9 mm
- net Net-(C3-Pad2): track 110.8 -> 0.00 mm, vias 1 -> 0
- net Net-(J18-PadT): track 0.00 -> 104.0 mm
- net Net-(C16-Pad1): track 0.00 -> 89.3 mm
- net +12V: track 411.3 -> 495.0 mm
- net Net-(J27-Pad3): track 0.00 -> 78.2 mm
- net Net-(J2-PadTN): track 0.00 -> 77.6 mm
- net Net-(C9-Pad2): track 74.7 -> 0.00 mm, vias 1 -> 0
- net Net-(J12-PadT): track 0.00 -> 74.1 mm
- net Net-(R47-Pad1): track 78.1 -> 5.97 mm
- net Net-(J2-PadT): track 0.00 -> 69.3 mm
- net Net-(J3-Pad1): track 0.00 -> 59.8 mm
- net /OSC2_LFO_Main: track 0.00 -> 57.4 mm
- net /I_FREQ: track 54.7 -> 0.00 mm
- net Net-(C18-Pad2): track 64.6 -> 13.9 mm
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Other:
- board size 143.8 x 103.8 mm -> 202 x 105 mm
- board text added: "Magnum Percussion Instrument rev 02"
- board text added: "This side towards panel"
- board text added: "output level"
- board text added: "piezo normalling"
- board text added: "piezo sensitivity"
- board text removed: "Filter Env Decay"
- board text removed: "Filter Freq"
- board text removed: "Filter LFO Mod"
- board text removed: "Freq CV"
- board text removed: "Freq Env"
- board text removed: "Magnum Percussion Instrument rev 01"
- board text removed: "Noise Level"
- board text removed: "OSC1 Freq"
- board text removed: "OSC1 Level"
- board text removed: "OSC2 Freq"
- board text removed: "OSC2 LFO"
- board text removed: "OSC2 Level"
- board text removed: "Out"
- board text removed: "Output Volume"
- board text removed: "Resonance"
- board text removed: "Trig"
- board text removed: "Volume Env CV"
- board text removed: "Volume Env Decay"
